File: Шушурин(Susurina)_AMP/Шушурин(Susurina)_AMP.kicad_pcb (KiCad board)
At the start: 2 copper layers, 120.7 x 85.1 mm, 58 parts

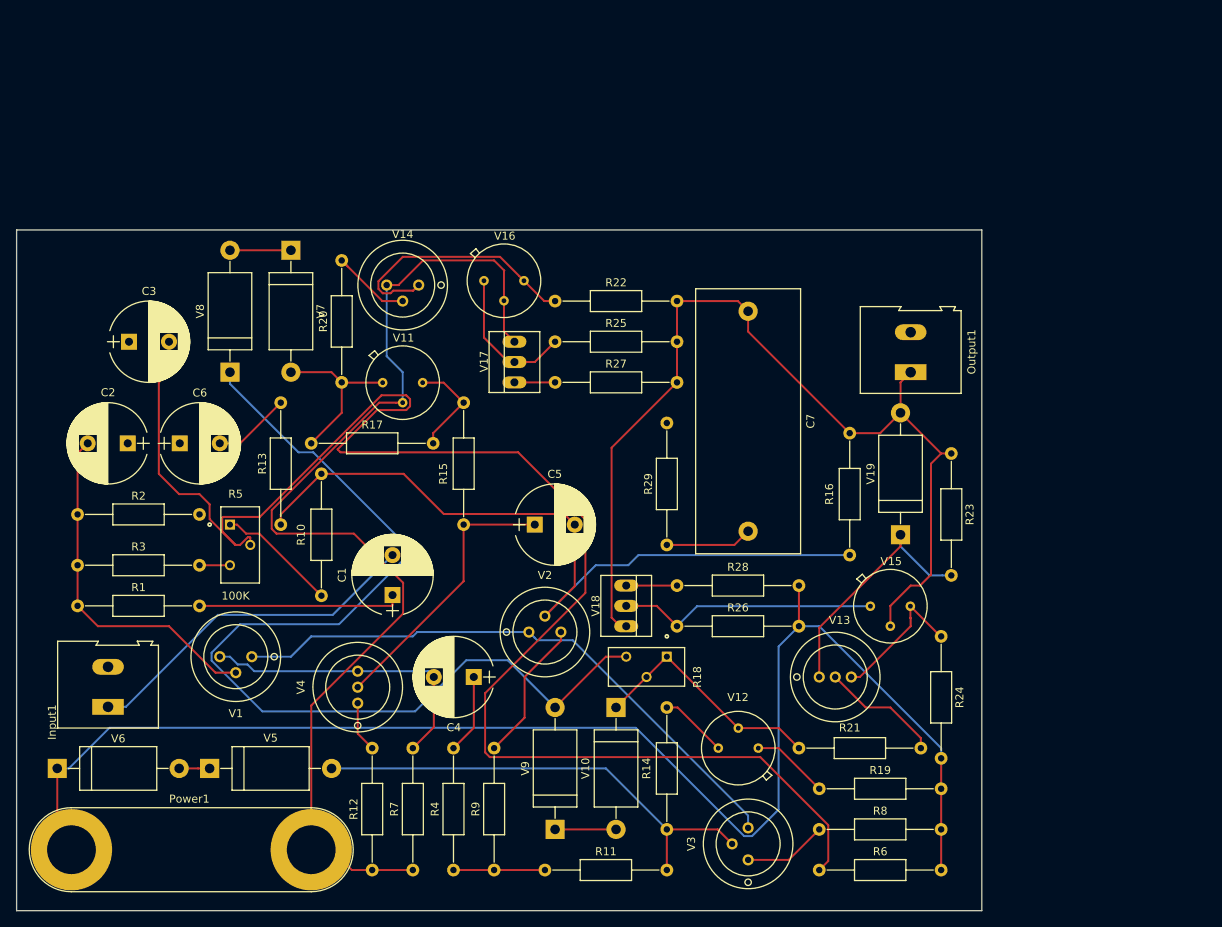
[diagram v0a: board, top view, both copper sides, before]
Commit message: 5.0
Gala darbs
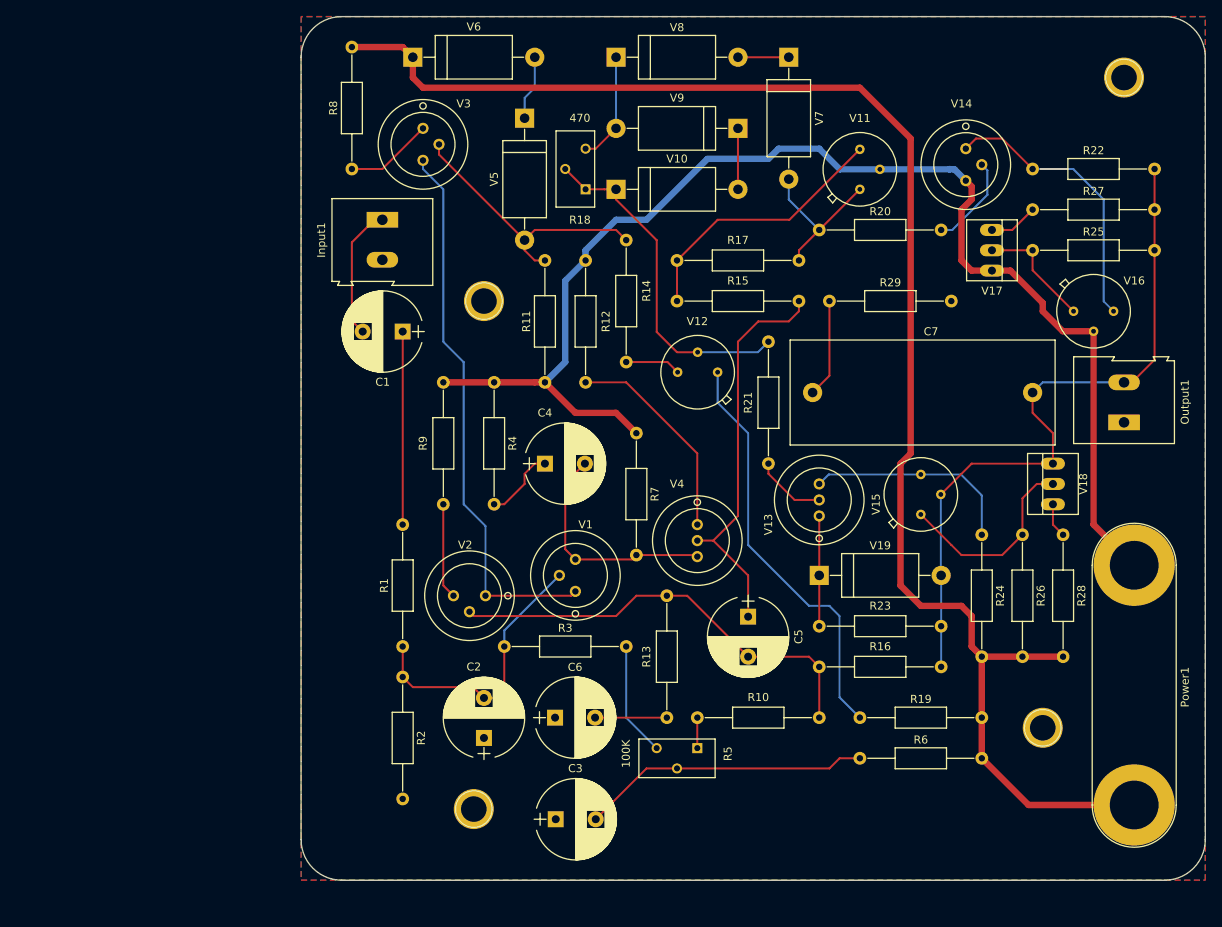
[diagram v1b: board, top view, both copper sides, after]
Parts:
- added REF**: 1pin, Connectors:1pin, F.Cu at (261.6, 33.0)
- added REF**: 1pin, Connectors:1pin, F.Cu at (251.5, 114.3)
- added REF**: 1pin, Connectors:1pin, F.Cu at (181.6, 61.0)
- added REF**: 1pin, Connectors:1pin, F.Cu at (180.3, 124.5)
- moved Power1 108.8 mm to (262.9, 94.0), turned to 270 degrees
- moved R8 101.1 mm to (165.1, 44.5), turned to 90 degrees
- moved V6 99.4 mm to (172.7, 30.5)
- moved V3 96.4 mm to (174.0, 41.4), turned to 270 degrees
- moved V9 90.6 mm to (213.4, 39.4), turned to 180 degrees
- moved V5 90.3 mm to (186.7, 38.1), turned to 270 degrees
- moved R12 80.7 mm to (194.3, 55.9), turned to 270 degrees
- moved C3 80.1 mm to (190.6, 125.7)
- moved V16 73.8 mm to (255.3, 62.2)
- moved V14 72.0 mm to (241.8, 43.9), turned to 270 degrees
- moved Input1 69.9 mm to (168.9, 50.8), turned to 270 degrees
- moved R10 69.3 mm to (223.5, 113.0), turned to 180 degrees
- moved V7 66.7 mm to (219.7, 30.5)
- moved R17 65.1 mm to (221.0, 55.9), turned to 180 degrees
- moved V10 64.8 mm to (198.1, 47.0), turned to 0 degrees
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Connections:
- Output1 pad 1: Net-(C7-Pad1) -> GNDD
- Output1 pad 2: GNDD -> Net-(C7-Pad1)
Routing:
- net Net-(C3-Pad2): track 202.5 -> 36.2 mm
- net Net-(R18-Pad3): track 125.4 -> 13.8 mm
- net Net-(R19-Pad1): track 9.72 -> 52.0 mm
- net Net-(C5-Pad2): track 97.0 -> 55.0 mm
- net Net-(C7-Pad1): track 121.5 -> 87.9 mm
- net Net-(C1-Pad2): track 43.4 -> 16.7 mm
- net Net-(R11-Pad2): track 59.1 -> 34.5 mm
- net Net-(R15-Pad1): track 12.8 -> 33.7 mm
- net Net-(R12-Pad2): track 6.37 -> 26.5 mm
- net Net-(R23-Pad2): track 31.3 -> 13.8 mm
- net Net-(C5-Pad1): track 34.7 -> 49.9 mm
- net +VDC: track 148.3 -> 162.8 mm
- net -VDC: track 178.5 -> 192.9 mm
- net Net-(R18-Pad1): track 30.2 -> 42.9 mm
- net Net-(R10-Pad2): track 15.1 -> 3.81 mm
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- added copper zone on B.Cu, net GNDD
- added copper zone on F.Cu, net GNDD
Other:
- board size 120.7 x 85.1 mm -> 113 x 108 mm
- net class +VDC added: clearance 0.2, trace_width 0.8, via_dia 0.6, via_drill 0.4
- net class -VDC added: clearance 0.2, trace_width 0.8, via_dia 0.6, via_drill 0.4
